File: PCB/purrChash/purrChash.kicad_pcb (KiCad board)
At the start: 2 copper layers, 39.5 x 70 mm, 28 parts, among them J1 USB4135-GF-A_REVA, M1 Motor_DC_ALT, Q1 Q_NMOS_GSD, U1 MSP430FR2110/MSP430FR2111, U2 MCP73811T-420I-OT, U3 TPS7A0533PDBZR

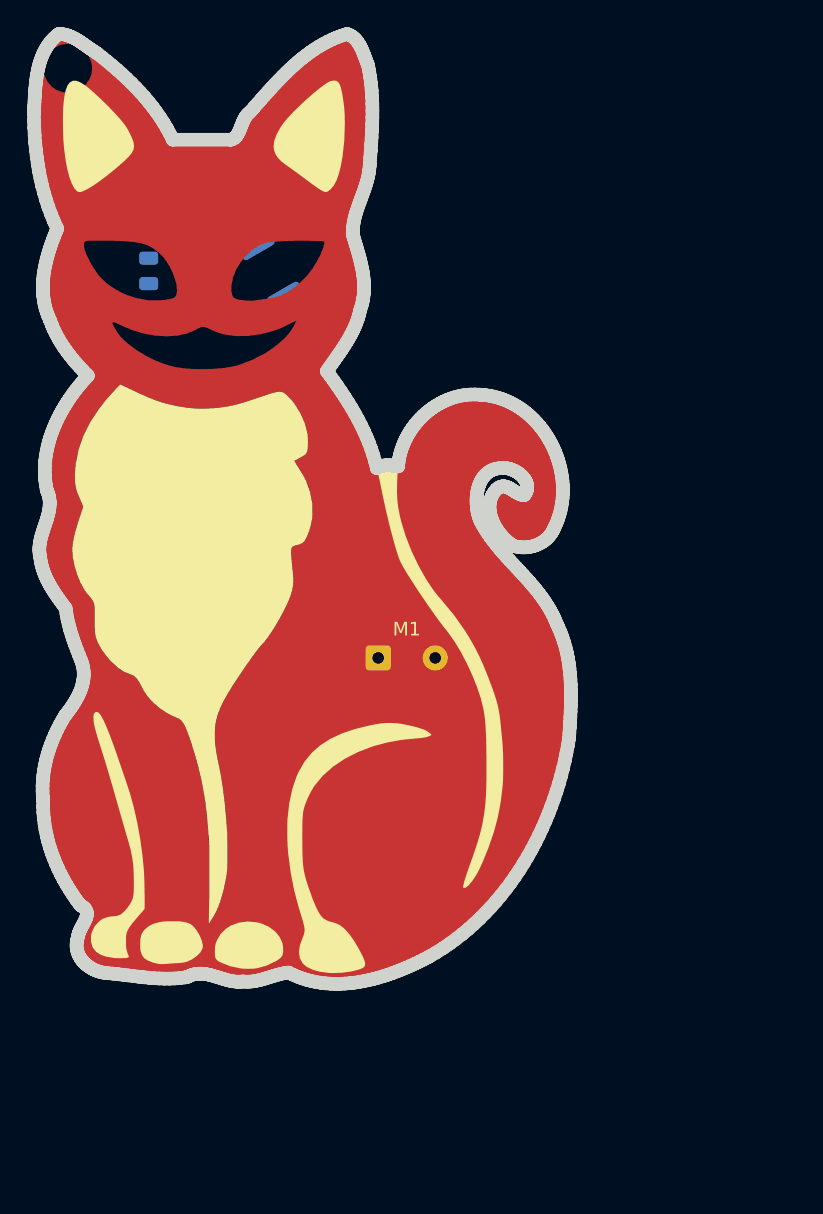
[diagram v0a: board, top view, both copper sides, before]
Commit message: more pcb work
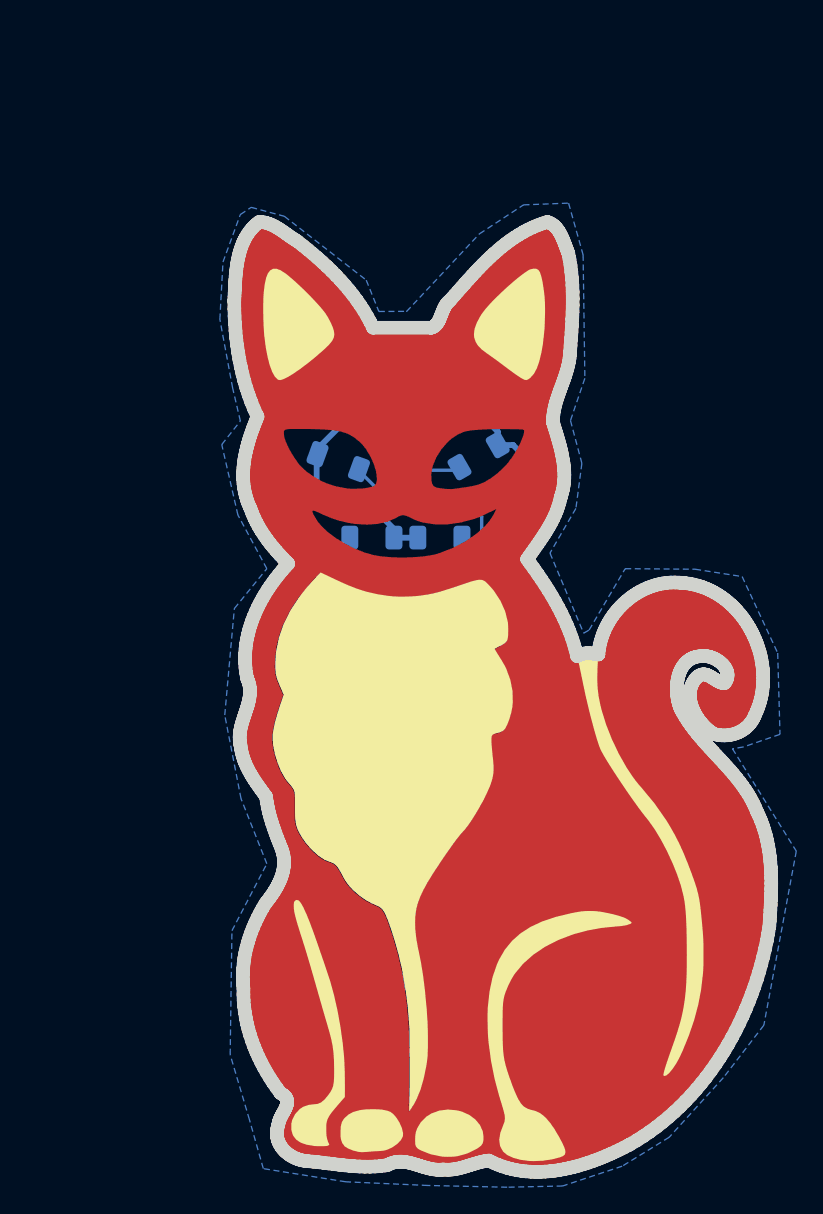
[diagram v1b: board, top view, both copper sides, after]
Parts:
- removed C7: 1u, Capacitor_SMD:C_0805_2012Metric
- added C6: 100n, Capacitor_SMD:C_0603_1608Metric, B.Cu at (43.1, 75.0)
- added D4: LED2, Library:LED_1206_3216Metric_shinethrough, B.Cu at (32.6, 31.2)
- added D5: LED3, Library:LED_1206_3216Metric_shinethrough, B.Cu at (24.7, 37.1)
- added D6: LED4, Library:LED_1206_3216Metric_shinethrough, B.Cu at (30.2, 37.1)
- added R10: 1k, Resistor_SMD:R_0603_1608Metric, B.Cu at (27.6, 32.2)
- added R11: 1k, Resistor_SMD:R_0603_1608Metric, B.Cu at (24.2, 39.3)
- added R12: 1k, Resistor_SMD:R_0603_1608Metric, B.Cu at (30.7, 39.3)
- added R7: 100k, Resistor_SMD:R_0603_1608Metric, B.Cu at (44.5, 64.0)
- added R8: 1k, Resistor_SMD:R_0603_1608Metric, B.Cu at (44.5, 65.5)
- added R9: 1k, Resistor_SMD:R_0603_1608Metric, B.Cu at (27.6, 33.7)
- added TP1: TouchPad, Connector_Wire:SolderWirePad_1x01_SMD_1x2mm, F.Cu at (26.4, 61.5)
- added TP2: TouchPad, Connector_Wire:SolderWirePad_1x01_SMD_1x2mm, F.Cu at (29.1, 55.2)
- added TP3: TouchPad, Connector_Wire:SolderWirePad_1x01_SMD_1x2mm, F.Cu at (22.8, 50.3)
- added TP4: TouchPad, Connector_Wire:SolderWirePad_1x01_SMD_1x2mm, F.Cu at (28.1, 45.9)
- C1, C2: value 10u -> 1u
- C3: value 100n -> 1u; footprint Capacitor_SMD:C_0603_1608Metric -> Capacitor_SMD:C_0805_2012Metric
- C4, C5: value 1u -> 10u
- D1: value D_Schottky -> CHG_LED; footprint Diode_SMD:D_0603_1608Metric -> LED_SMD:LED_0603_1608Metric
- D2: value LED -> D_Schottky; footprint LED_SMD:LED_2010_5025Metric_Pad1.52x2.65mm_HandSolder -> Diode_SMD:D_0603_1608Metric
- D3: value LED -> LED1; footprint LED_SMD:LED_0805_2012Metric -> Library:LED_1206_3216Metric_shinethrough
- M1: moved to B.Cu
- R1: value 100k -> 5.1k
- R2, R3, R4: value 1k -> 5.1k
- R6: value 5.1k -> 1k
- U1: value MSP430FR2110/MSP430FR2111 -> BQ21040DBV; footprint Package_SO:TSSOP-16_4.4x5mm_P0.65mm -> Package_TO_SOT_SMD:SOT-23-6
- U2: value MCP73811T-420I-OT -> TPS7A0533PDBZR
- U3: value TPS7A0533PDBZR -> MSP430FR2110/MSP430FR2111; footprint Package_TO_SOT_SMD:SOT-23-5 -> Package_SO:TSSOP-16_4.4x5mm_P0.65mm
- moved R2 52.8 mm to (35.1, 77.2), turned to 90 degrees
- moved D2 48.6 mm to (39.7, 60.7), turned to -90 degrees
- moved R3 48.1 mm to (30.8, 73.1)
- moved C4 36.9 mm to (43.1, 76.8), turned to 180 degrees
- moved U2 28.5 mm to (37.7, 73.6)
- moved U3 27.3 mm to (43.6, 70.2), turned to 90 degrees
- moved C5 26.3 mm to (41.7, 60.9)
- moved C2 25.3 mm to (34.8, 73.4)
- moved R1 24.6 mm to (20.4, 77.2)
- moved C3 21.4 mm to (37.7, 76.7), turned to 0 degrees
- moved D1 21.2 mm to (31.5, 69.5), turned to 0 degrees
- moved J1 20.2 mm to (27.8, 79.4)
- moved ? 20.2 mm to (14.8, 13.8) (x2)
- moved ? 20.2 mm to (14.7, 13.9)
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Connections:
- C1 pad 1: /3V3 -> /5V_USB
- C2 pad 1: /3V3 -> /VBAT
- C4 pad 1: /5V_USB -> /3V3
- C5 pad 1: /VBAT -> /3V3
- D1 pad 1: /3V3 -> CHG
- D1 pad 2: GND -> /CHG_LED
- D2 pad 1: /LED1_R -> /3V3
- D2 pad 2: /3V3 -> GND
- D3 pad 1: /LED2_R -> /LED1_R
- R1 pad 1: /MOTOR_MCU_R -> /CC2
- R2 pad 1: /LED1_R -> /CC1
- R2 pad 2: /LED_MCU -> GND
- R3 pad 1: /LED2_R -> /ISET
- R3 pad 2: /LED_MCU -> GND
- R4 pad 1: /MOTOR_MCU_R -> /TS
- R4 pad 2: /MOTOR_MCU -> /TS_R
- R5 pad 1: /CC2 -> /TS_R
- R6 pad 1: /CC1 -> /VBAT
- R6 pad 2: GND -> /CHG_LED
- U1 pad 1: unconnected-(U1-P1.1/UCA0CLK/ACLK/C1/A1-Pad1) -> /TS
- U1 pad 2: unconnected-(U1-P1.0/UCA0STE/SMCLK/C0/A1/Veref+-Pad2) -> /VBAT
- U1 pad 3: unconnected-(U1-TEST/SBWTCK-Pad3) -> CHG
- U1 pad 4: unconnected-(U1-NRST/NMI/SBWTDIO-Pad4) -> /ISET
- U1 pad 5: /3V3 -> GND
- U1 pad 6: GND -> /5V_USB
- U2 pad 1: /5V_USB -> /VBAT
- U2 pad 4: /5V_USB -> unconnected-(U2-NC-Pad4)
- U2 pad 5: GND -> /3V3
- U3 pad 1: /VBAT -> unconnected-(U3-P1.1/UCA0CLK/ACLK/C1/A1-Pad1)
- U3 pad 2: GND -> unconnected-(U3-P1.0/UCA0STE/SMCLK/C0/A1/Veref+-Pad2)
- U3 pad 3: /VBAT -> unconnected-(U3-TEST/SBWTCK-Pad3)
- U3 pad 4: unconnected-(U3-NC-Pad4) -> CHG
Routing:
- net /3V3: track 0.00 -> 118.5 mm
- net /LED_MCU1: track 0.00 -> 43.1 mm
- net /LED_MCU2: track 0.00 -> 37.7 mm
- net Net-(U3-P1.5/UCA0CLK/TMS/A5): track 0.00 -> 34.0 mm, vias 0 -> 1
- net Net-(U3-P1.6/UCA0RXD/UCA0SOMI/TB0.1/TDI/TCLK/A6): track 0.00 -> 32.0 mm, vias 0 -> 1
- net Net-(U3-P1.4/UCA0STE/TCK/A4): track 0.00 -> 24.9 mm, vias 0 -> 1
- net Net-(U3-P1.3/UCA0STE/TCK/A4): track 0.00 -> 24.2 mm, vias 0 -> 1
- net /VBAT: track 0.00 -> 21.5 mm
- net CHG: track 0.00 -> 19.4 mm
- net GND: track 0.00 -> 14.8 mm
- net /5V_USB: track 0.00 -> 8.11 mm
- net /CC2: track 0.00 -> 7.98 mm
- net /CC1: track 0.00 -> 7.90 mm
- net /LED1_R: track 0.00 -> 3.64 mm
- net /MOTOR_MCU_R: track 0.00 -> 3.31 mm
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- added copper zone on B.Cu, net GND
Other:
- outline, holes or cut-outs redrawn
- board text added: "&"
- board text added: "GalH"
- board text added: "TalyR"
